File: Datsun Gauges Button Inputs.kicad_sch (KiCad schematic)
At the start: 14 parts, among them SW1 SW_Push, SW2 SW_Push, U1 4049, U2 4049

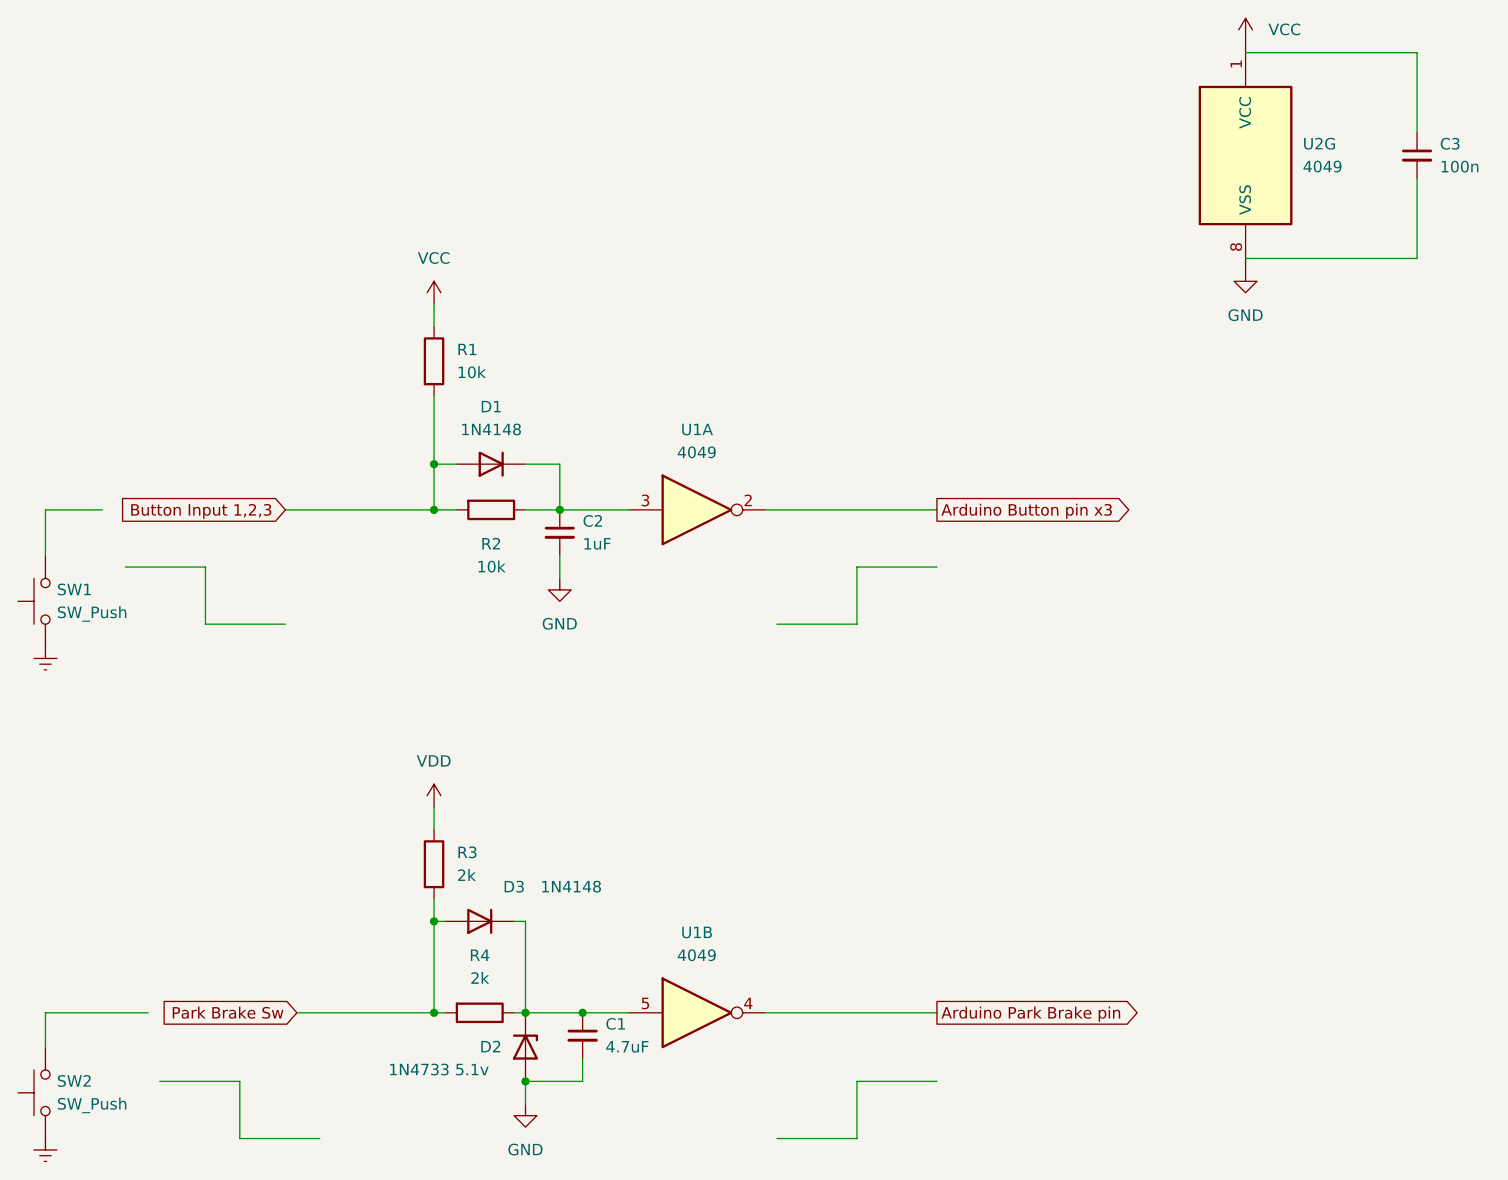
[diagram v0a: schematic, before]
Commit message: Cleanup
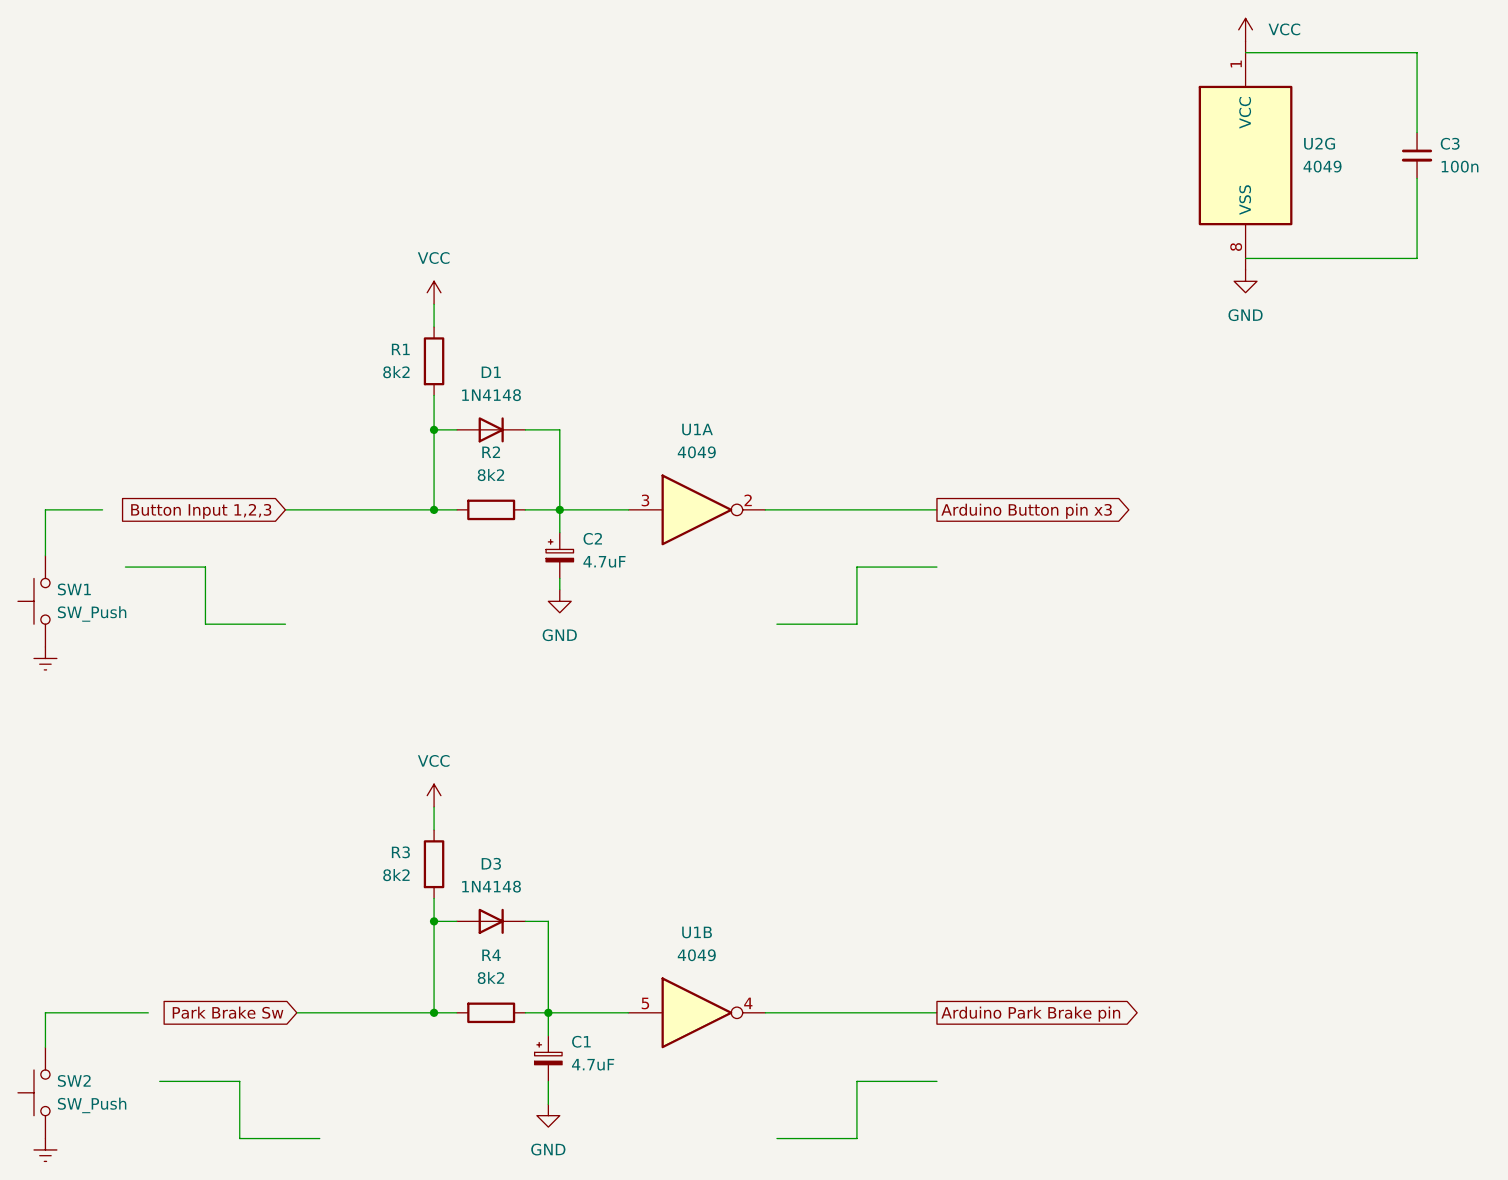
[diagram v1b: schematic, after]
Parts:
- removed C1: 4.7uF, symbol Device:C_Small
- removed C2: 1uF, symbol Device:C_Small
- removed D2: 1N4733 5.1v, Diode_THT:D_DO-41_SOD81_P10.16mm_Horizontal, symbol Diode:1N47xxA
- added C1, C2: 4.7uF, symbol Device:C_Polarized_Small
- R1, R2: value 10k -> 8k2
- R3, R4: value 2k -> 8k2
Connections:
- net VDD is gone; now on net VCC: R3.1
- net GND: now also C1.2, C2.2
- net at D3.1 (K), R4.1, U1.5: now also C1.1
- net at D1.1 (K), R2.1, U1.3: now also C2.1
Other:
- moved on the sheet: D1, D3, R4
